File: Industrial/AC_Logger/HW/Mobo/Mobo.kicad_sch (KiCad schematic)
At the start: 4 parts, among them J1 Conn_01x11_Female

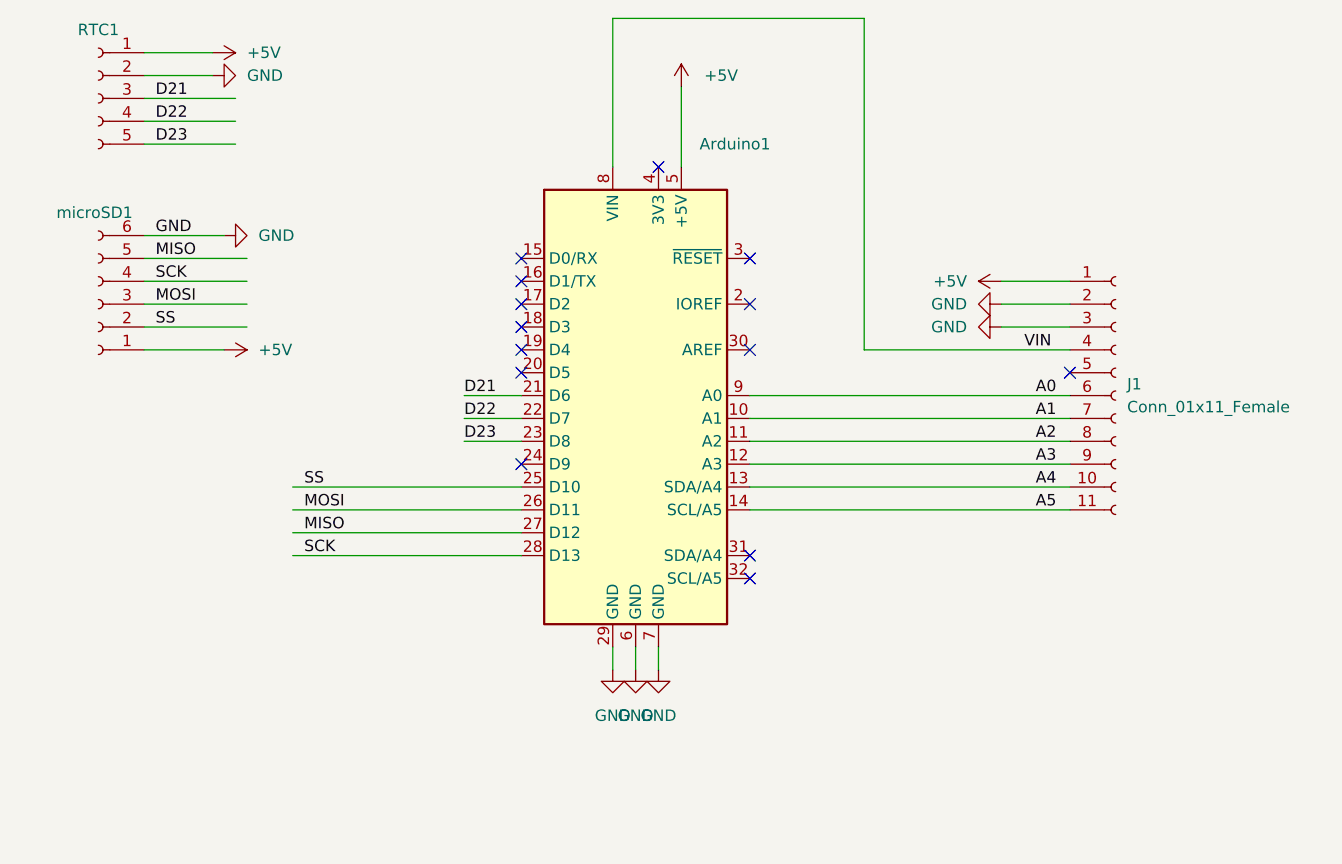
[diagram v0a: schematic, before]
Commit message: Finising touches on PCB and Schematic
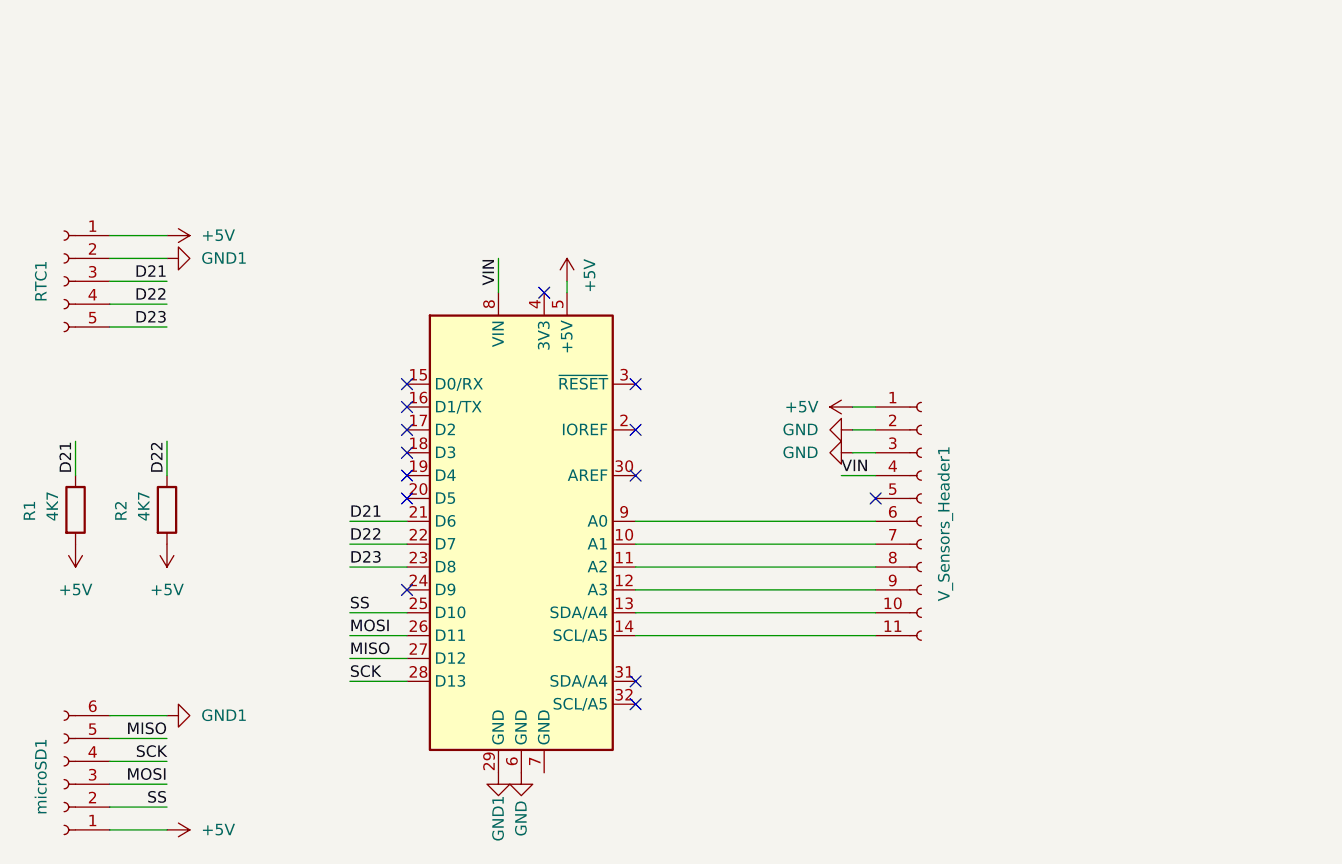
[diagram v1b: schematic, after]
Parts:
- added R1, R2: 4K7, Resistor_THT:R_Axial_DIN0207_L6.3mm_D2.5mm_P7.62mm_Horizontal, symbol Device:R
- renumbered J1 to V_Sensors_Header1
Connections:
- net +5V: now also R1.2, R2.2
- net D21: now also R1.1
- net D22: now also R2.1
- net GND: no longer Arduino1.29 (GND), Arduino1.7 (GND), RTC1.2 (Pin_2), microSD1.6 (Pin_6)
- net A0: no longer names the net of Arduino1.9 (A0), V_Sensors_Header1.6 (Pin_6)
- net A1: no longer names the net of Arduino1.10 (A1), V_Sensors_Header1.7 (Pin_7)
- net A2: no longer names the net of Arduino1.11 (A2), V_Sensors_Header1.8 (Pin_8)
- net A3: no longer names the net of Arduino1.12 (A3), V_Sensors_Header1.9 (Pin_9)
- net A4: no longer names the net of Arduino1.13 (SDA/A4), V_Sensors_Header1.10 (Pin_10)
- net A5: no longer names the net of Arduino1.14 (SCL/A5), V_Sensors_Header1.11 (Pin_11)
- new net GND1: Arduino1.29 (GND), RTC1.2 (Pin_2), microSD1.6 (Pin_6)
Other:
- moved on the sheet: RTC1, V_Sensors_Header1, microSD1
